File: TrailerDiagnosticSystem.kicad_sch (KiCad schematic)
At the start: 2 parts, among them J3 Conn_01x10, J4 Conn_01x10

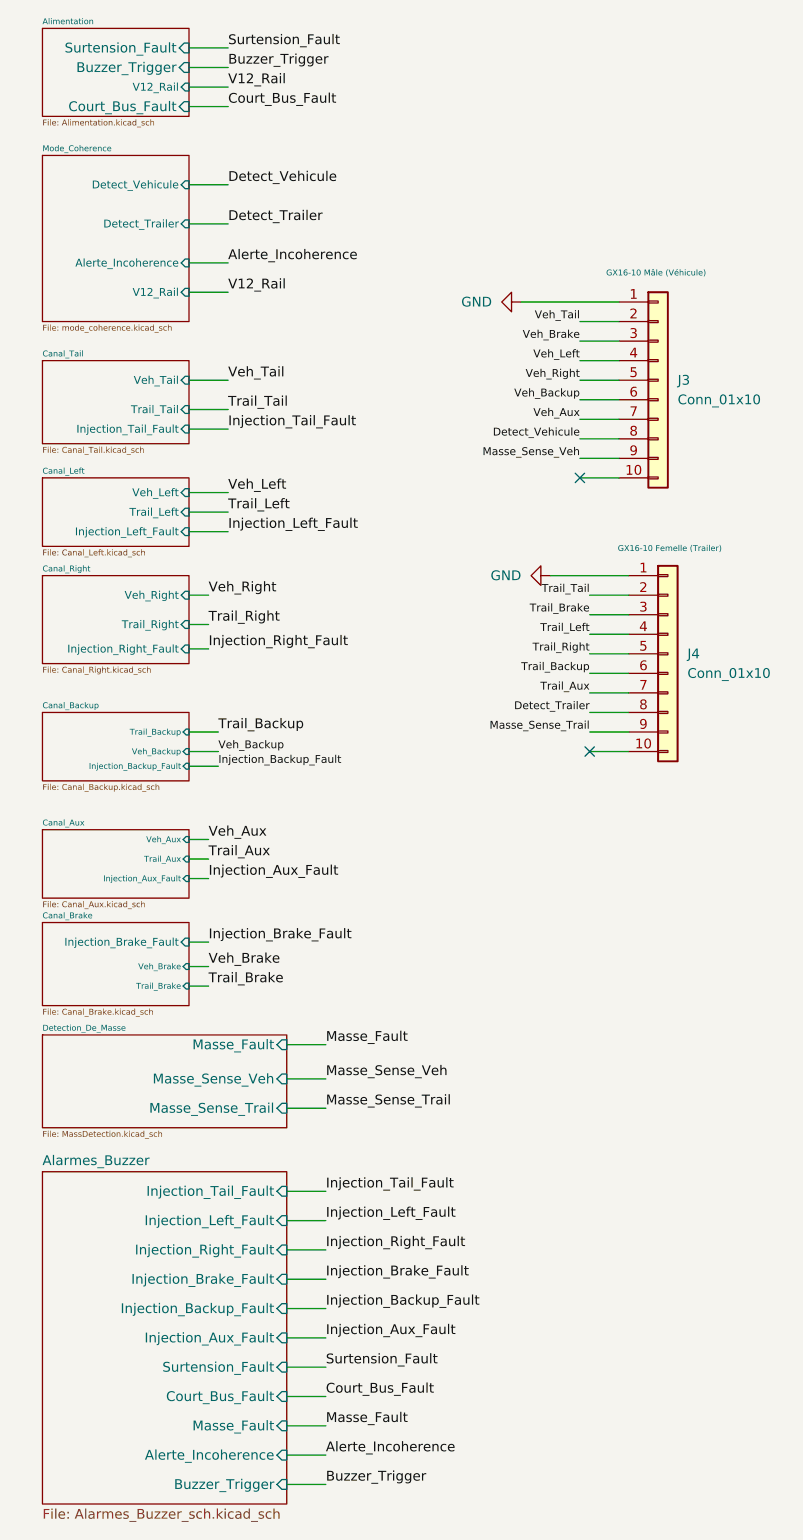
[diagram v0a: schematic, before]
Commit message: Add files via upload
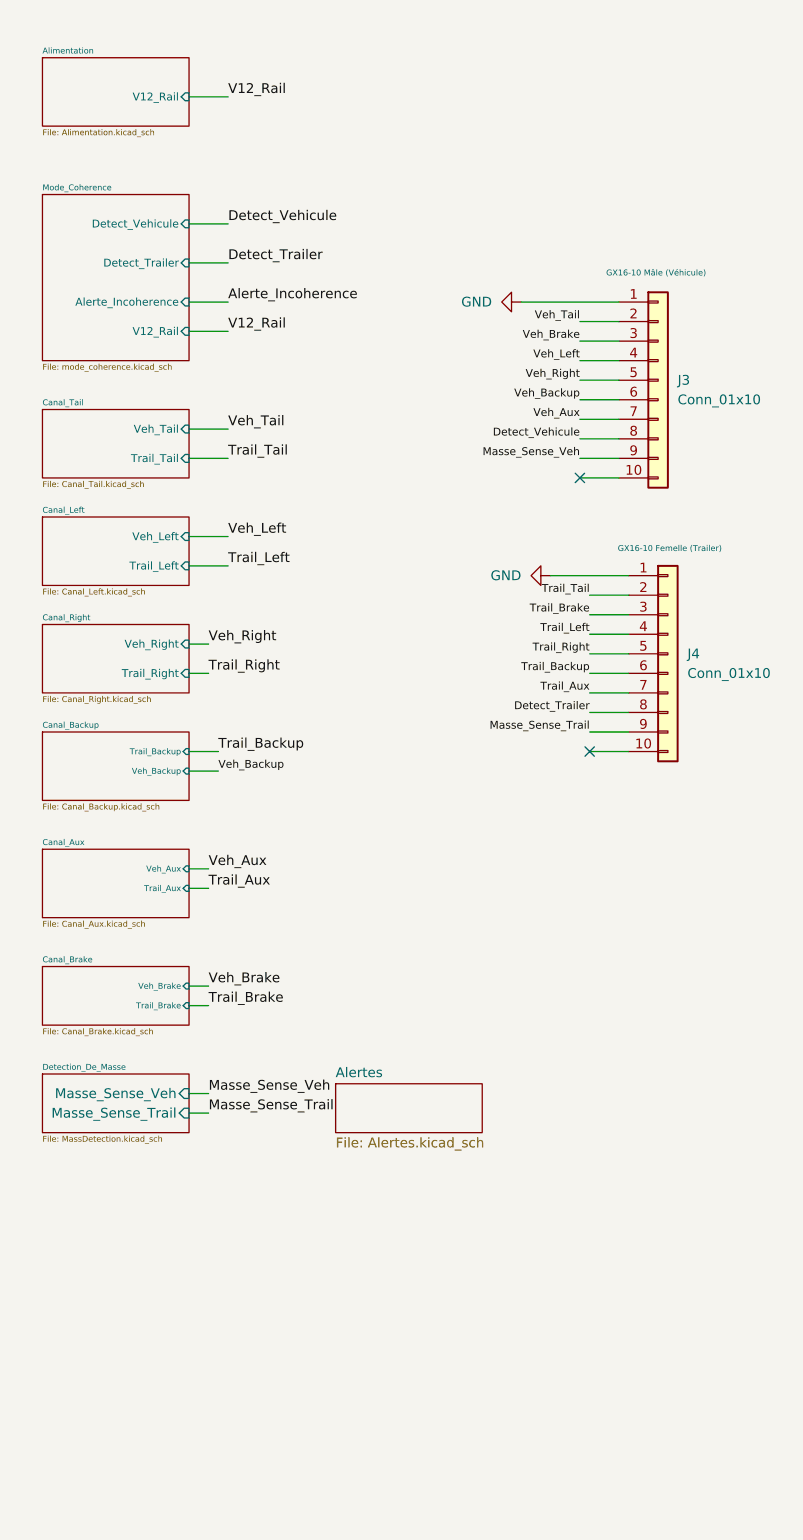
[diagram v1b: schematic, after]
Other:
- sheet Alarmes_Buzzer renamed Alertes
- sheet Alertes: file Alarmes_Buzzer_sch.kicad_sch -> Alertes.kicad_sch
- sheet Alertes ports: added none; removed Alerte_Incoherence, Buzzer_Trigger, Court_Bus_Fault, Injection_Aux_Fault, Injection_Backup_Fault, Injection_Brake_Fault, Injection_Left_Fault, Injection_Right_Fault, Injection_Tail_Fault, Masse_Fault, Surtension_Fault
- sheet Alimentation ports: added none; removed Buzzer_Trigger, Court_Bus_Fault, Surtension_Fault
- sheet Canal_Aux ports: added none; removed Injection_Aux_Fault
- sheet Canal_Backup ports: added none; removed Injection_Backup_Fault
- sheet Canal_Brake ports: added none; removed Injection_Brake_Fault
- sheet Canal_Left ports: added none; removed Injection_Left_Fault
- sheet Canal_Right ports: added none; removed Injection_Right_Fault
- sheet Canal_Tail ports: added none; removed Injection_Tail_Fault
- sheet Detection_De_Masse ports: added none; removed Masse_Fault
